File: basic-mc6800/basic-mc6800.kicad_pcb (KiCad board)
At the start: 2 copper layers, 100 x 45 mm, 32 parts, among them J1 Conn_01x39_Male, J2 Conn_01x04_Male, U1 74LV32, U2 MC6809, U3 IS61C256AL, U4 28C256, U5 74LV14, Y1 ABLS-4.000MHZ-20-B-3-H-T

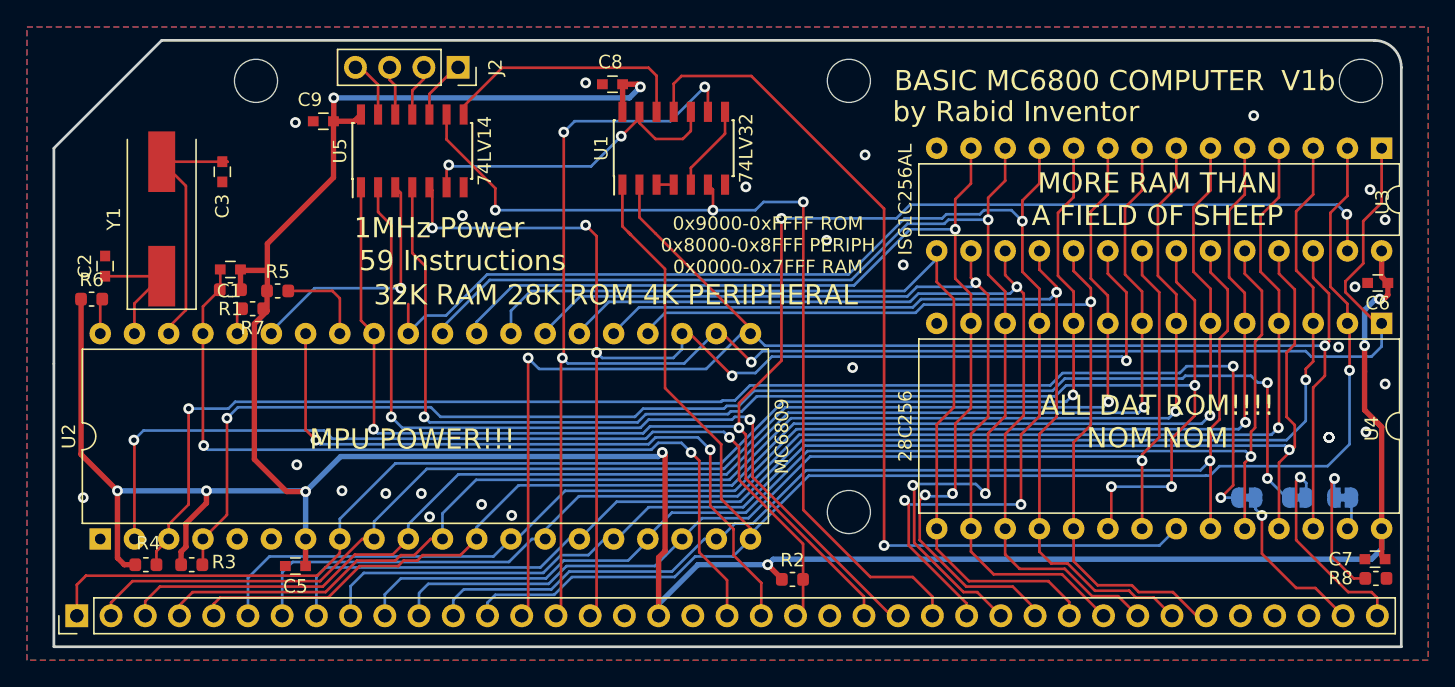
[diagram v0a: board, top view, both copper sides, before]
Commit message: final tweaks and created gerber
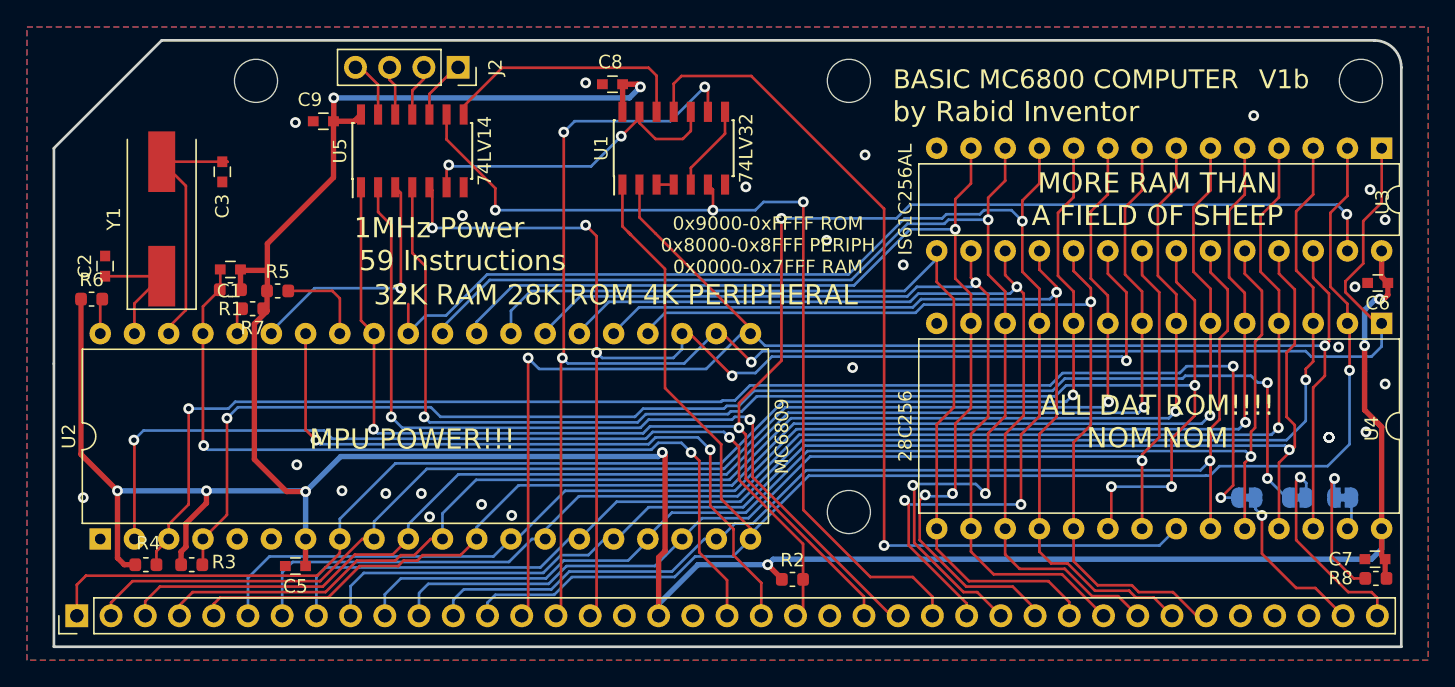
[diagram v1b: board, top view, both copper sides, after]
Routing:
- net +5V: track 238.6 -> 240.1 mm
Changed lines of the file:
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@@
   (general
     (thickness 1.6)
-    (drawings 29)
-    (tracks 926)
+    (drawings 28)
+    (tracks 928)
     (zones 0)
     (modules 32)
@@
       (drillshape 0)
       (scaleselection 1)
-      (outputdirectory "mc6800_v1_0gerber/"))
+      (outputdirectory "mc6800_v1_bgerber/"))
   )
   (net 0 "")
@@
     (effects (font (size 0.7 0.7) (thickness 0.1)) (justify mirror))
   )
-  (gr_text V1b (at 191.1 60) (layer F.SilkS)
-    (effects (font (size 1.5 1.5) (thickness 0.3)))
+  (gr_text V1b (at 189.3 59.9) (layer F.SilkS)
+    (effects (font (size 1.4 1.4) (thickness 0.3)))
   )
   (dimension 15 (width 0.3) (layer F.Fab)
@@
     (arrow2b (pts (xy 84.1 60) (xy 84.686421 61.126504)))
   )
-  (target plus (at 98 102) (size 5) (width 0.15) (layer Edge.Cuts))
   (gr_line (start 98 65) (end 106 57) (layer Edge.Cuts) (width 0.2))
   (gr_text "MORE RAM THAN \nA FIELD OF SHEEP" (at 179.9 68.8) (layer F.SilkS)
@@
     (effects (font (size 1.5 1.5) (thickness 0.3)))
   )
-  (gr_text "BASIC MC6800 COMPUTER\n" (at 174.1 60) (layer F.SilkS)
-    (effects (font (size 1.5 1.5) (thickness 0.3)))
+  (gr_text "BASIC MC6800 COMPUTER\n" (at 173.1 59.9) (layer F.SilkS)
+    (effects (font (size 1.4 1.4) (thickness 0.3)))
   )
   (dimension 100 (width 0.3) (layer F.Fab)
@@
   (segment (start 100.0125 87.7189) (end 102.7176 90.424) (width 0.4) (layer F.Cu) (net 4))
   (segment (start 100.0125 76.2) (end 100.0125 87.7189) (width 0.4) (layer F.Cu) (net 4))
+  (segment (start 196.8 96.8256) (end 196.9008 96.9264) (width 0.4) (layer F.Cu) (net 4))
+  (segment (start 196.8 95.5) (end 196.8 96.8256) (width 0.4) (layer F.Cu) (net 4))
   (segment (start 99.7 99.7) (end 99.7 97.404) (width 0.2) (layer F.Cu) (net 5))
   (segment (start 99.7 97.404) (end 100.3808 96.7232) (width 0.2) (layer F.Cu) (net 5))
